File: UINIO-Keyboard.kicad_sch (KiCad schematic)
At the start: 93 parts, among them J1 Conn_01x06_Pin, J2 Conn_01x05_Pin, J3 Conn_01x05_Pin, K1 A, K10 A, K11 A, K12 A, K13 A, K14 A, K15 A, K16 A, K17 A, K18 A, K19 A, K2 A, K20 A, K21 A, K22 A, K23 A, K24 A, K25 A, K26 A, K27 A, K28 A, K29 A, K3 A, K30 A, K31 A, K32 A, K33 A, K34 A, K35 A, K36 A, K37 A, K38 A, K39 A, K4 A, K40 A, K41 A, K42 A, K43 A, K44 A, K45 A, K46 A, K47 A, K48 A, K49 A, K5 A, K50 A, K51 A, K52 A, K53 A, K54 A, K55 A, K56 A, K57 A, K58 A, K59 A, K6 A, K60 A, K61 A, K62 A, K63 A, K64 A, K7 A, K8 A, K9 A, U1 CH452A, U2 EC1106S, U3 EC1106S

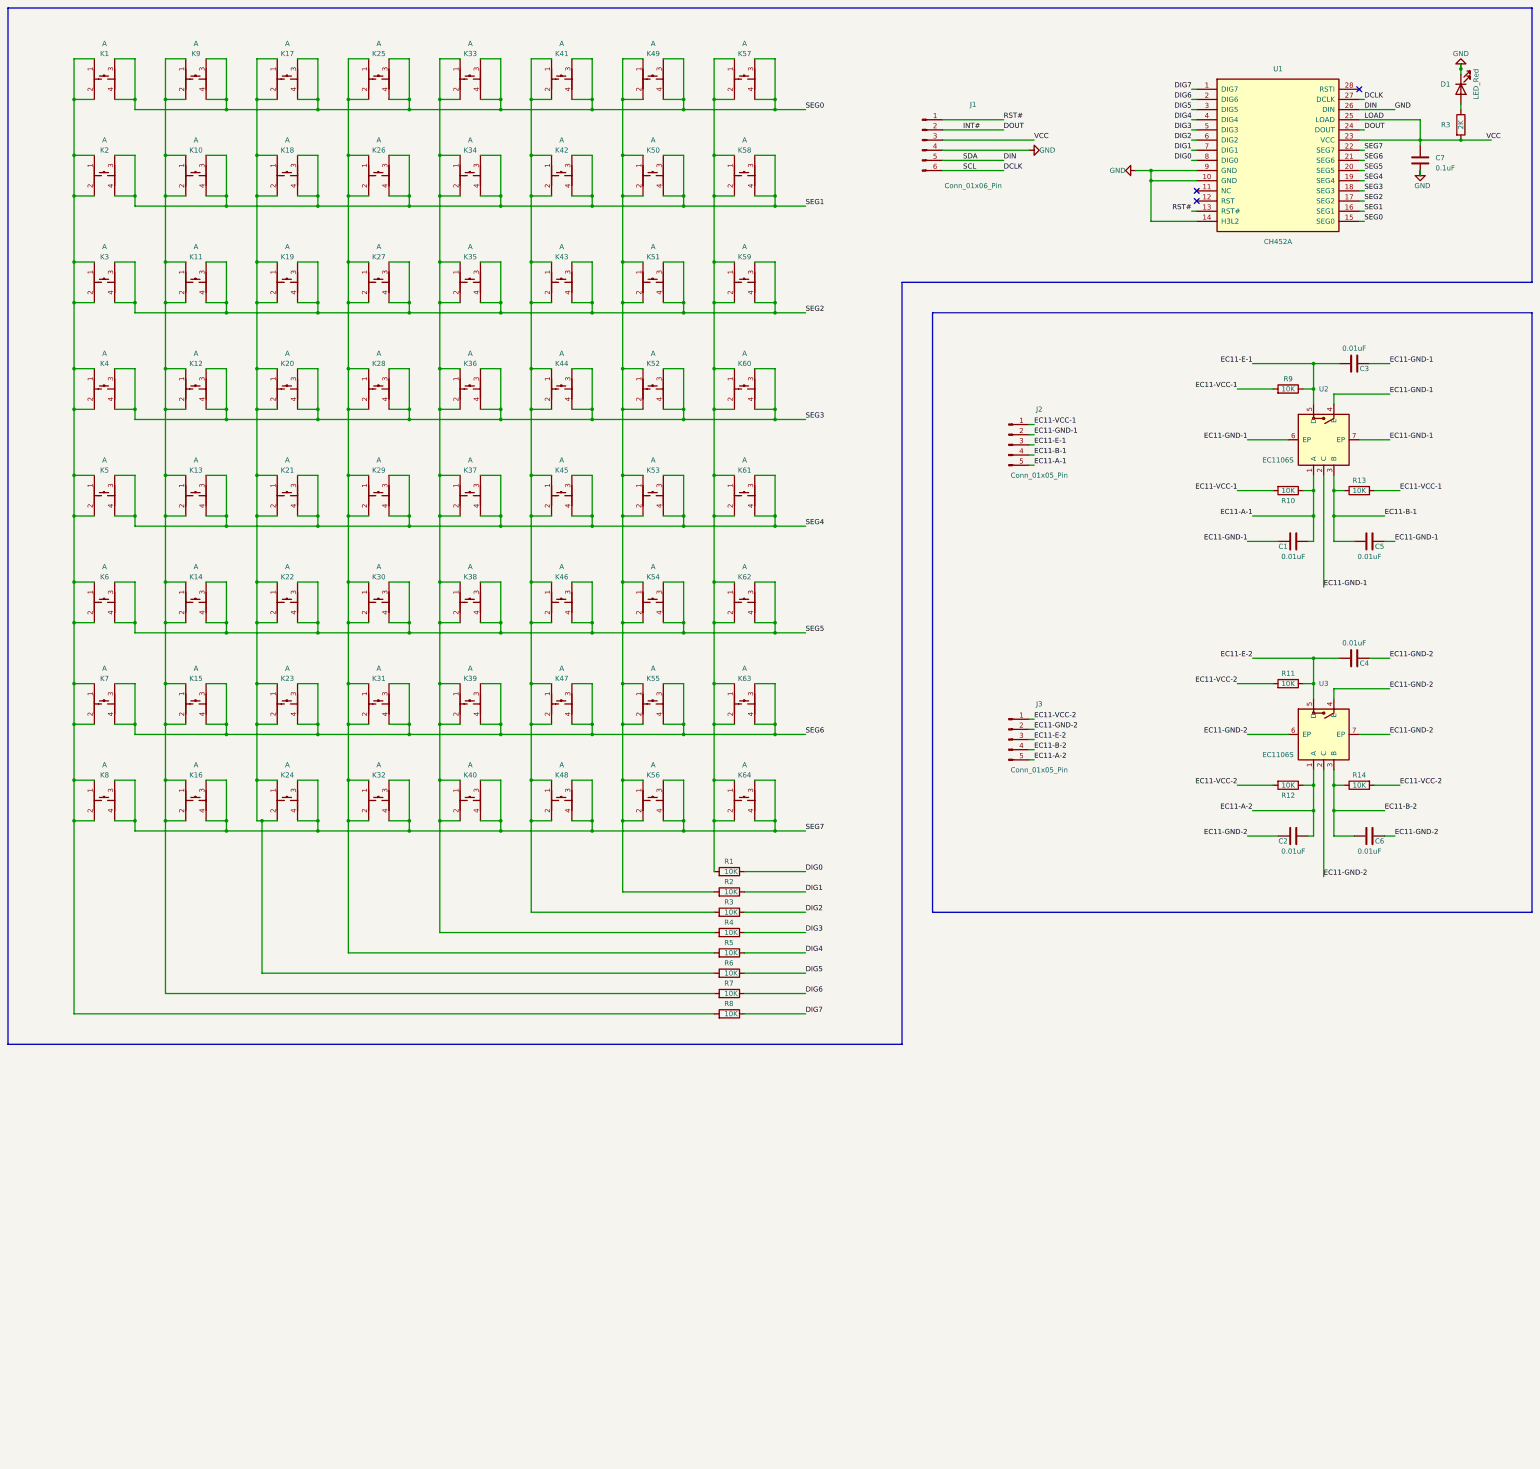
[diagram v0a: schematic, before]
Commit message: PCB Layout.
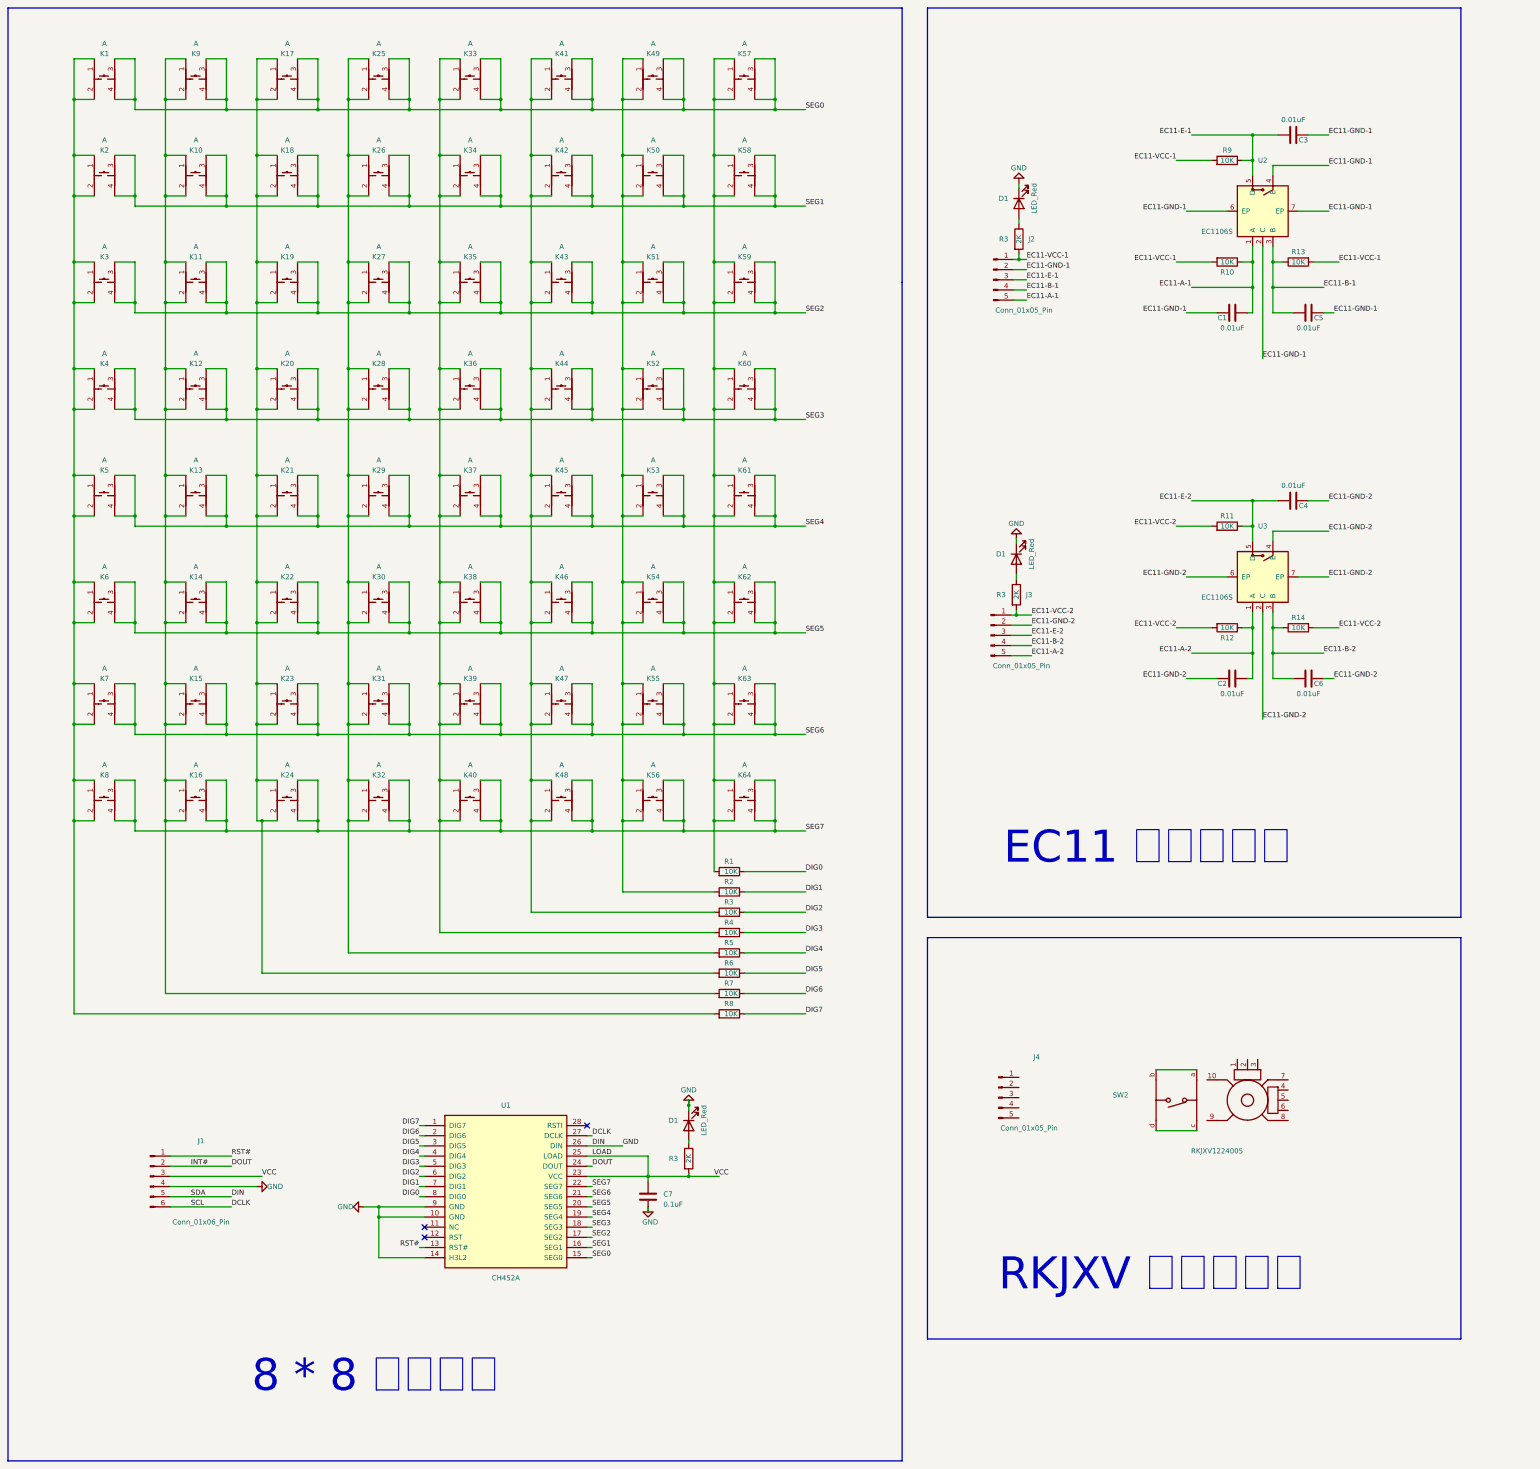
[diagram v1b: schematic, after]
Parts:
- added D1 (x2): LED_Red, LED_SMD:LED_0603_1608Metric, symbol Device:LED
- added J4: Conn_01x05_Pin, Connector_PinHeader_2.54mm:PinHeader_1x05_P2.54mm_Vertical, symbol Connector:Conn_01x05_Pin
- added R3 (x2): 2K, Resistor_SMD:R_0402_1005Metric, symbol Device:R
- added SW2: RKJXV1224005, Uinio:SW-TH_RKJXV1224005, symbol Uinio:RKJXV1224005
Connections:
- net EC11-VCC-1: now also R3.2
- net EC11-VCC-2: now also R3.2
- net GND: now also D1.1 (K), D1.1 (K)
- new net: D1.2 (A), R3.1 (x2)
- new net: SW2.a, SW2.b
- new net: SW2.c, SW2.d
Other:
- note added: "8 * 8 矩阵键盘"
- note added: "EC11 旋转编码器"
- note added: "RKJXV 模拟量摇杆"
- moved on the sheet: C1, C2, C3, C4, C5, C6, C7, D1, J1, J2, J3, R10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
